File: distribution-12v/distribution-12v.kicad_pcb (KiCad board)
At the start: 2 copper layers, 37.5 x 67.5 mm, 11 parts, among them J1 Conn_01x02_Socket, J2 Conn_01x02_Socket, J3 Conn_01x02_Socket, J4 Conn_01x02_Socket, J5 Conn_01x02_Socket

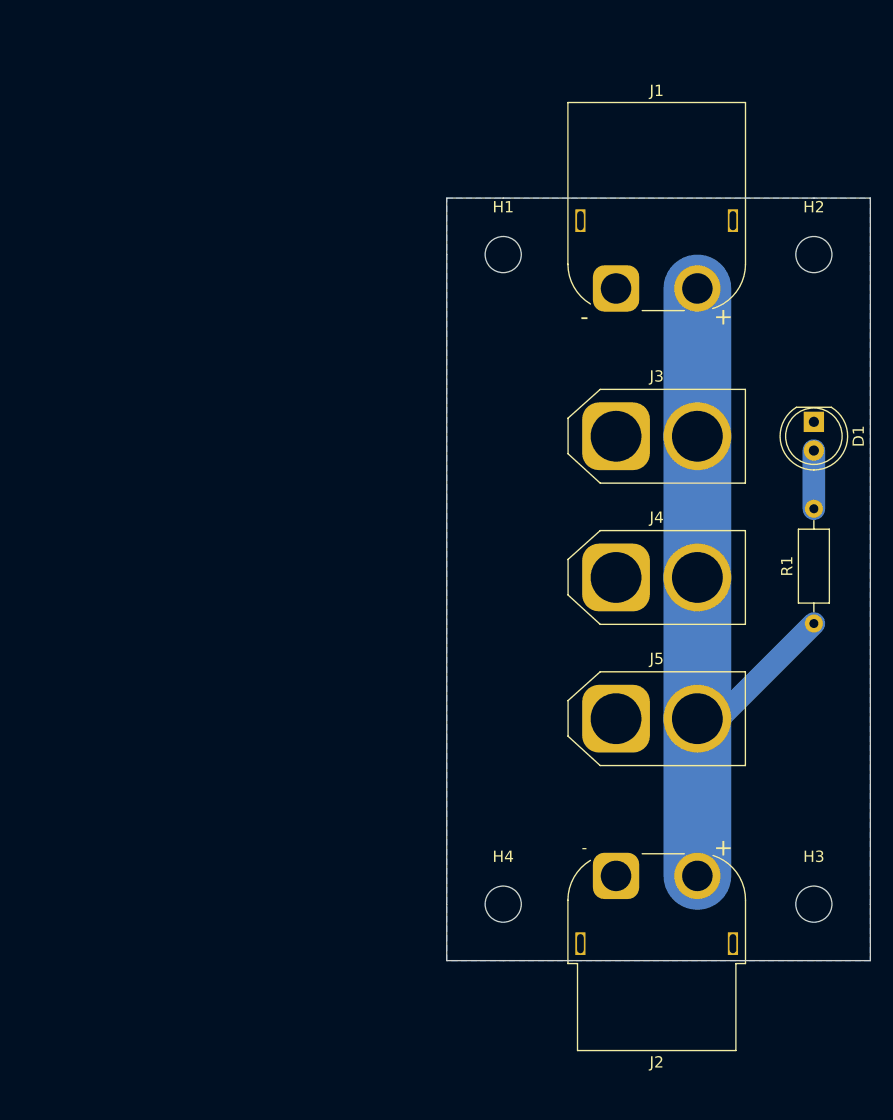
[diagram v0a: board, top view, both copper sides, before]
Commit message: fix: まるごと作り直し
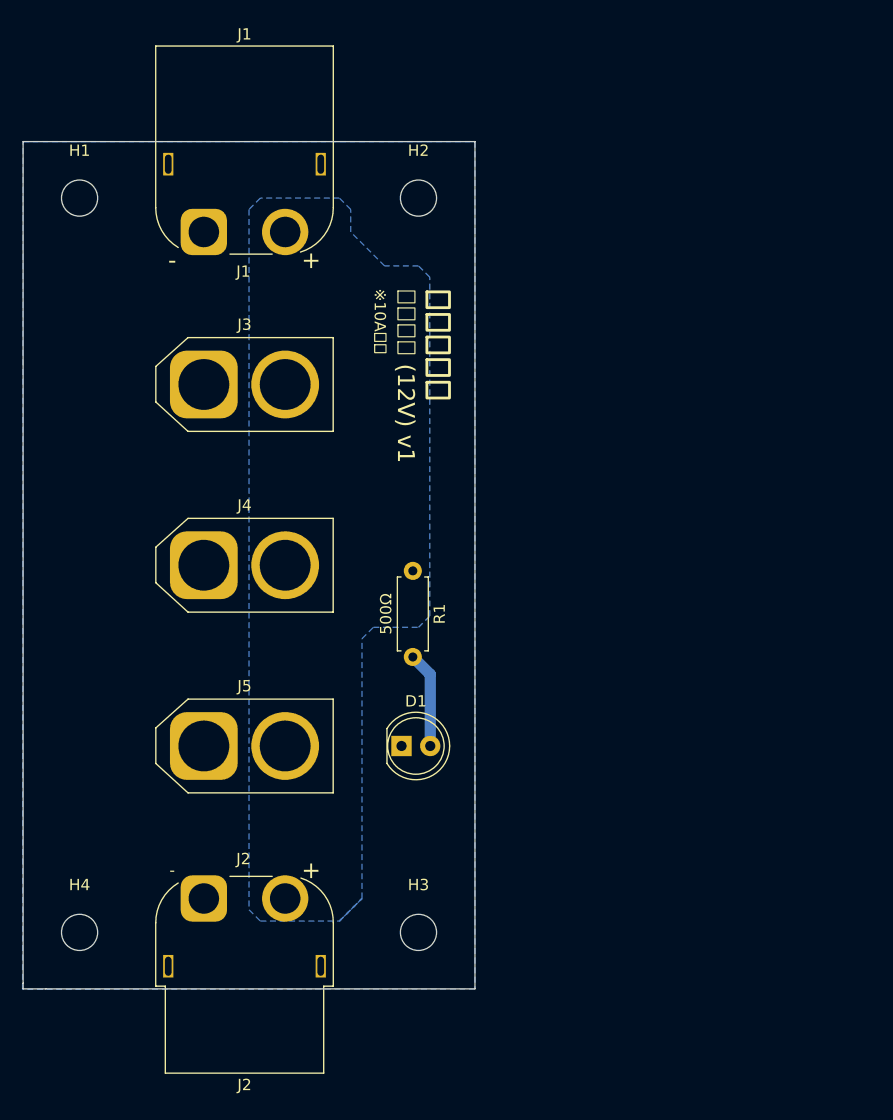
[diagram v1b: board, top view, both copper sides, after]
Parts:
- R1: footprint Resistor_THT:R_Axial_DIN0207_L6.3mm_D2.5mm_P10.16mm_Horizontal -> Resistor_THT:R_Axial_DIN0207_L6.3mm_D2.5mm_P7.62mm_Horizontal
- moved D1 46.4 mm to (108.5, 93.5), turned to 0 degrees
- moved H1 37.8 mm to (80.0, 45.0)
- moved H4 37.6 mm to (80.0, 110.0)
- moved J1 36.8 mm to (91.0, 48.0)
- moved J3 36.8 mm to (91.0, 61.5)
- moved J5 36.6 mm to (91.0, 93.5)
- moved J2 36.5 mm to (91.0, 107.0)
- moved J4 36.5 mm to (91.0, 77.5)
- moved R1 35.8 mm to (109.5, 78.0), turned to -90 degrees
- moved H2 35.4 mm to (110.0, 45.0)
- moved H3 35.1 mm to (110.0, 110.0)
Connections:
- J1 pad : (no net) -> GND
- J2 pad : (no net) -> GND
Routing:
- net +12V: track 65.8 -> 0.00 mm
- net Net-(D1-A): track 5.15 -> 8.52 mm
- added copper zone on B.Cu, net +12V
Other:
- board size 37.5 x 67.5 mm -> 40 x 75 mm
- board text added: "※10Aまで"
- board text added: "新居浜高専"
- board text added: "配電基盤 (12V) v1"
